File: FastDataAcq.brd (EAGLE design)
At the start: 114.3 x 62.7 mm, 215 parts, among them IC1 LT1963AEQ, IC2 FT230XQ, IC3 ADCMP553BRMZ, J1 MICRO-FIT_3.0_2POS_RA_SMD, J2 USB_MICROAB_SMT, X1 87832-14, X2 SMA-142-0701-801/806, X3 SMA-142-0701-801/806, Y1 SI530-500, Y2 100MHz, Y3 DNP

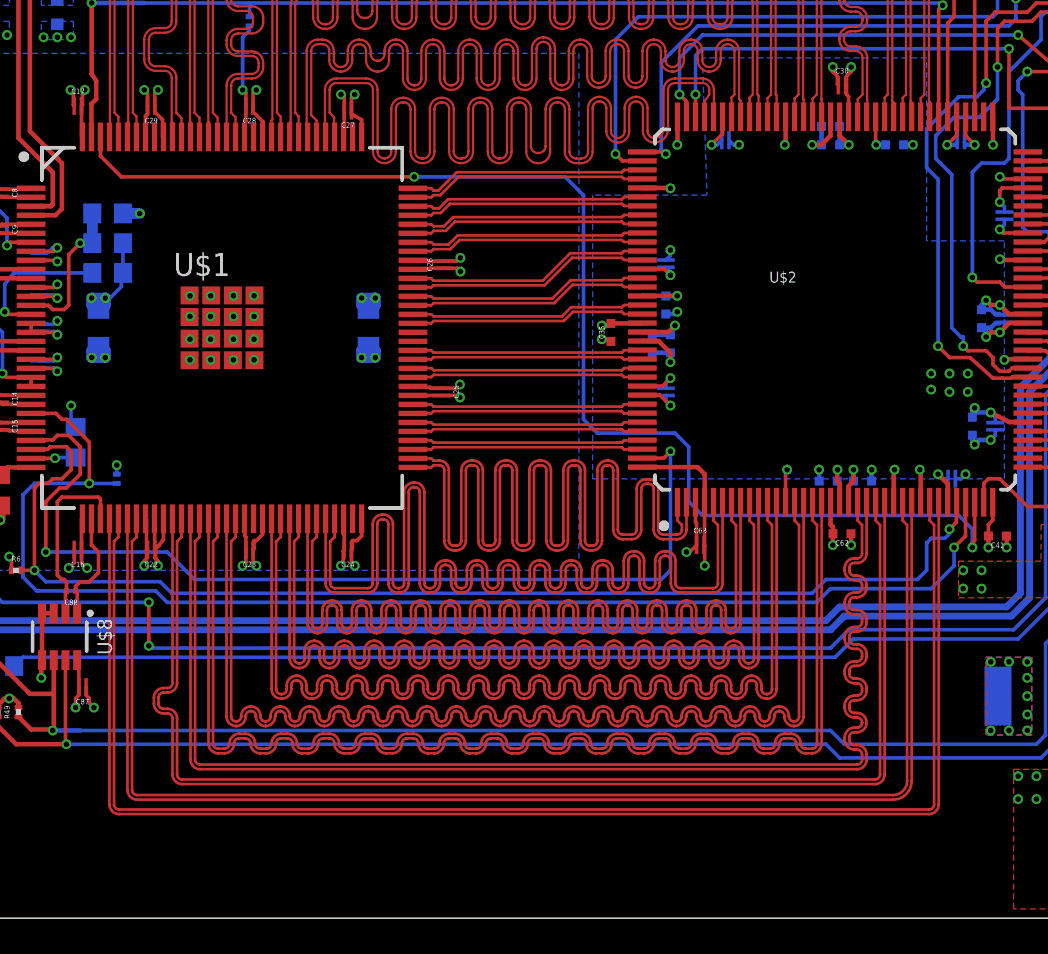
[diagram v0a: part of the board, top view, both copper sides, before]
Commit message: Partially done with LVDS bottom half.
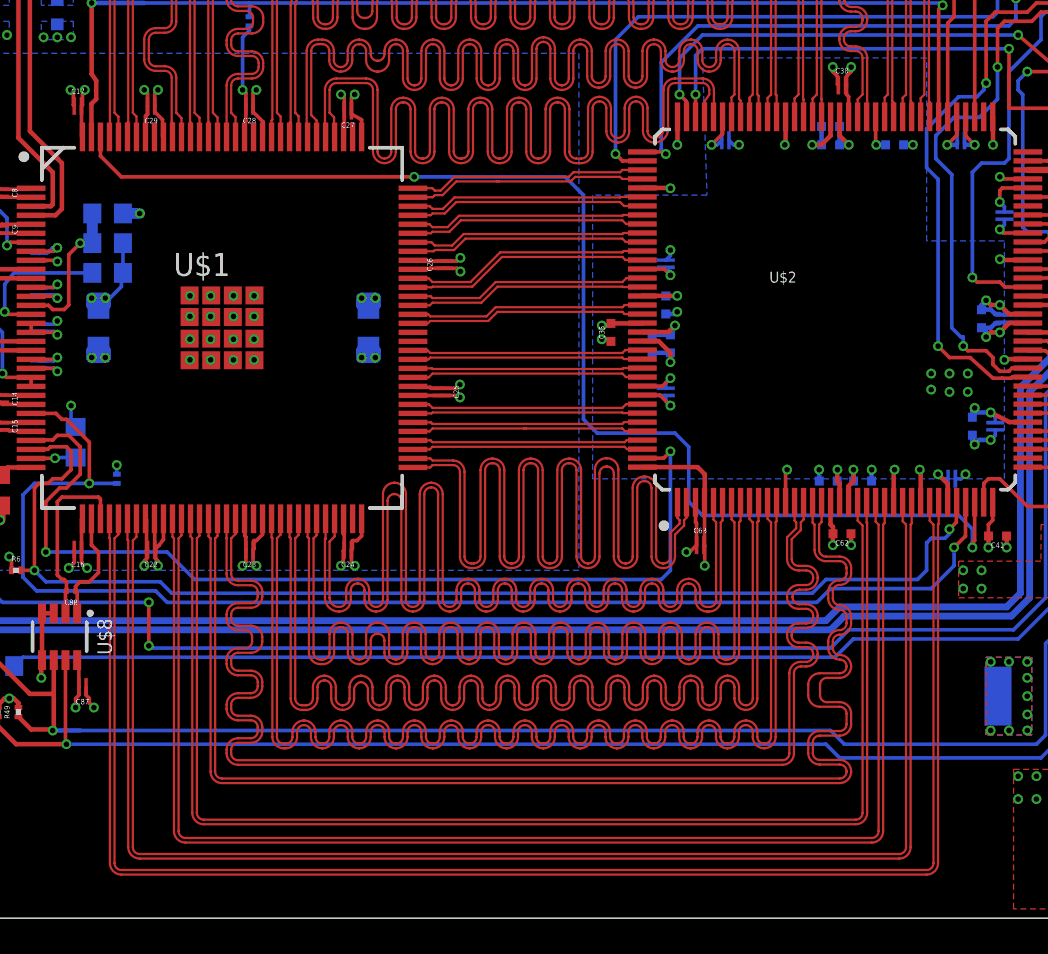
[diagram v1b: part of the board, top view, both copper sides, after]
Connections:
- net DQ0+ renamed DQ0_P
- net DQ0- renamed DQ0_N
- net DQ1+ renamed DQ1_P
- net DQ1- renamed DQ1_N
- net DQ2+ renamed DQ2_P
- net DQ2- renamed DQ2_N
- net DQD0+ renamed DQD0_P
- net DQD0- renamed DQD0_N
- net DQD1+ renamed DQD1_P
- net DQD1- renamed DQD1_N
- net DQD2+ renamed DQD2_P
- net DQD2- renamed DQD2_N
- net DQD3+ renamed DQD3_P
- net DQD3- renamed DQD3_N
- net DQD4+ renamed DQD4_P
- net DQD4- renamed DQD4_N
- net DQD5+ renamed DQD5_P
- net DQD5- renamed DQD5_N
- net DQD6+ renamed DQD6_P
- net DQD6- renamed DQD6_N
- net DQD7+ renamed DQD7_P
- net DQD7- renamed DQD7_N
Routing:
- net DQD1_P: track 74.7 -> 81.4 mm
- net DQD1_N: track 74.2 -> 80.8 mm
- net DQD0_P: track 79.1 -> 85.7 mm
- net DQD0_N: track 78.6 -> 85.1 mm
- net DQD6_P: track 65.6 -> 71.6 mm
- net DQD7_N: track 65.8 -> 71.8 mm
- net DQD6_N: track 65.0 -> 71.0 mm
- net DQD7_P: track 66.3 -> 72.2 mm
- net DQ1_N: track 67.1 -> 72.4 mm
- net DQD2_P: track 70.4 -> 75.6 mm
- net DQ2_N: track 68.1 -> 73.2 mm
- net DQ0_N: track 66.6 -> 71.6 mm
- net DQD2_N: track 69.9 -> 74.9 mm
- net DQ2_P: track 68.3 -> 73.2 mm
- net DQ1_P: track 67.6 -> 72.4 mm
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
